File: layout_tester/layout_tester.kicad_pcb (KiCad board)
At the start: 2 copper layers, 178.4 x 118.1 mm, 31 parts, among them SW1 SW_Push

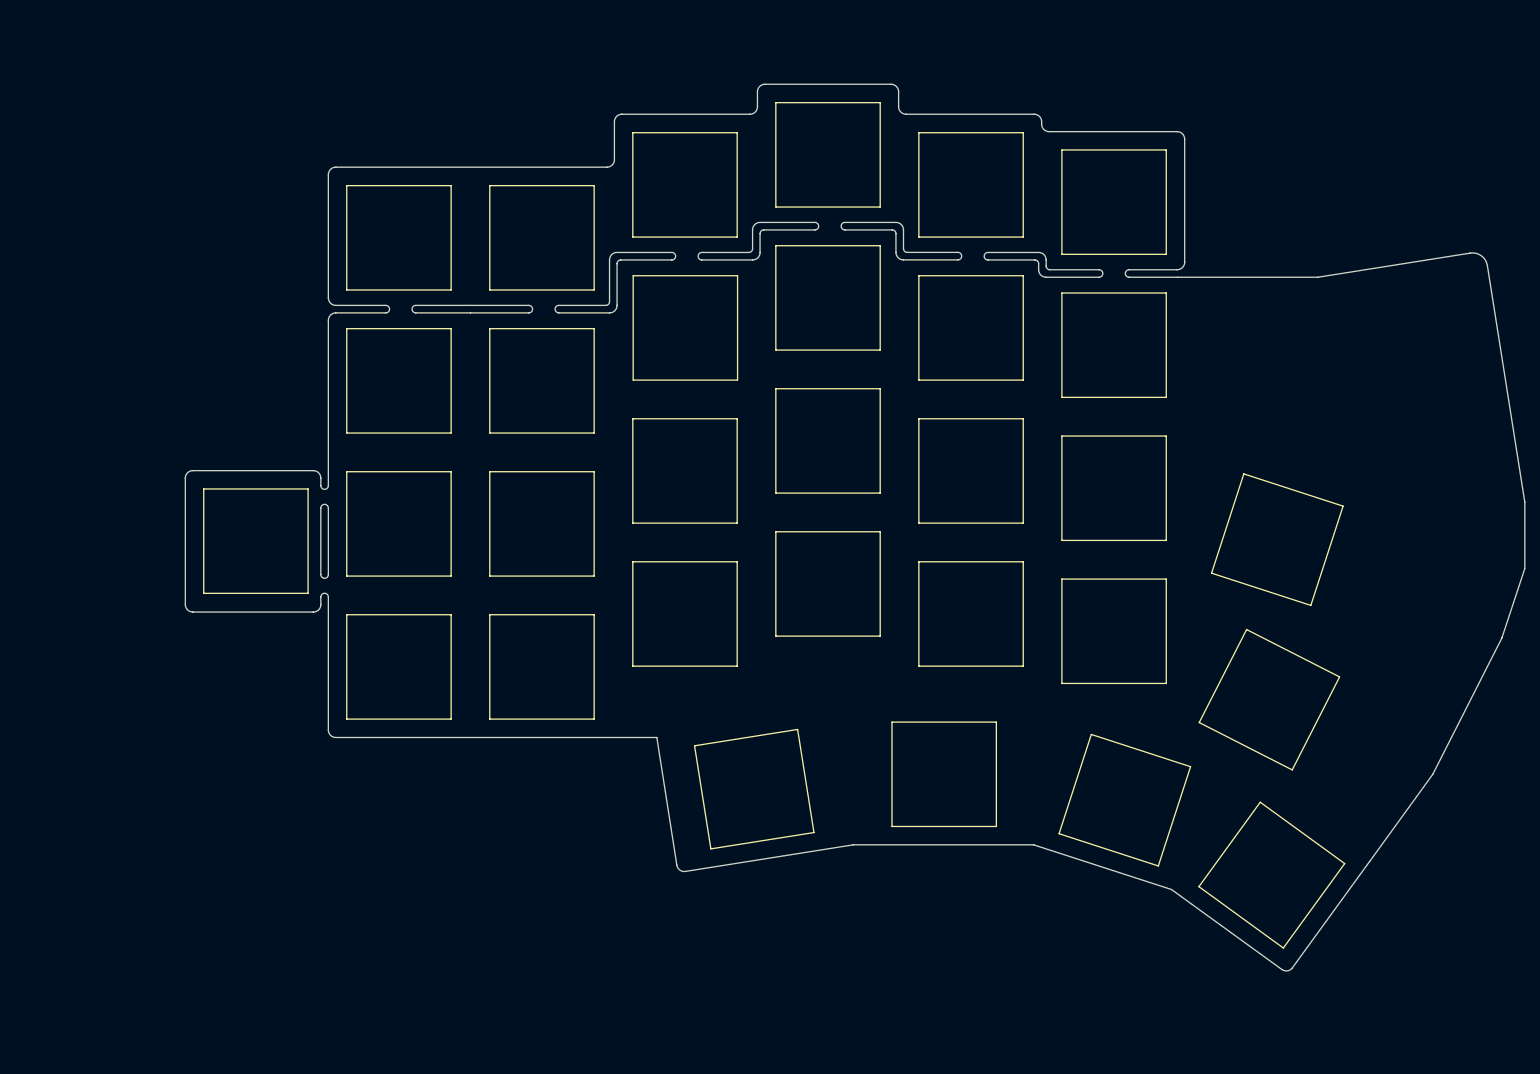
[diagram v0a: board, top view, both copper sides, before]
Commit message: Layout tester
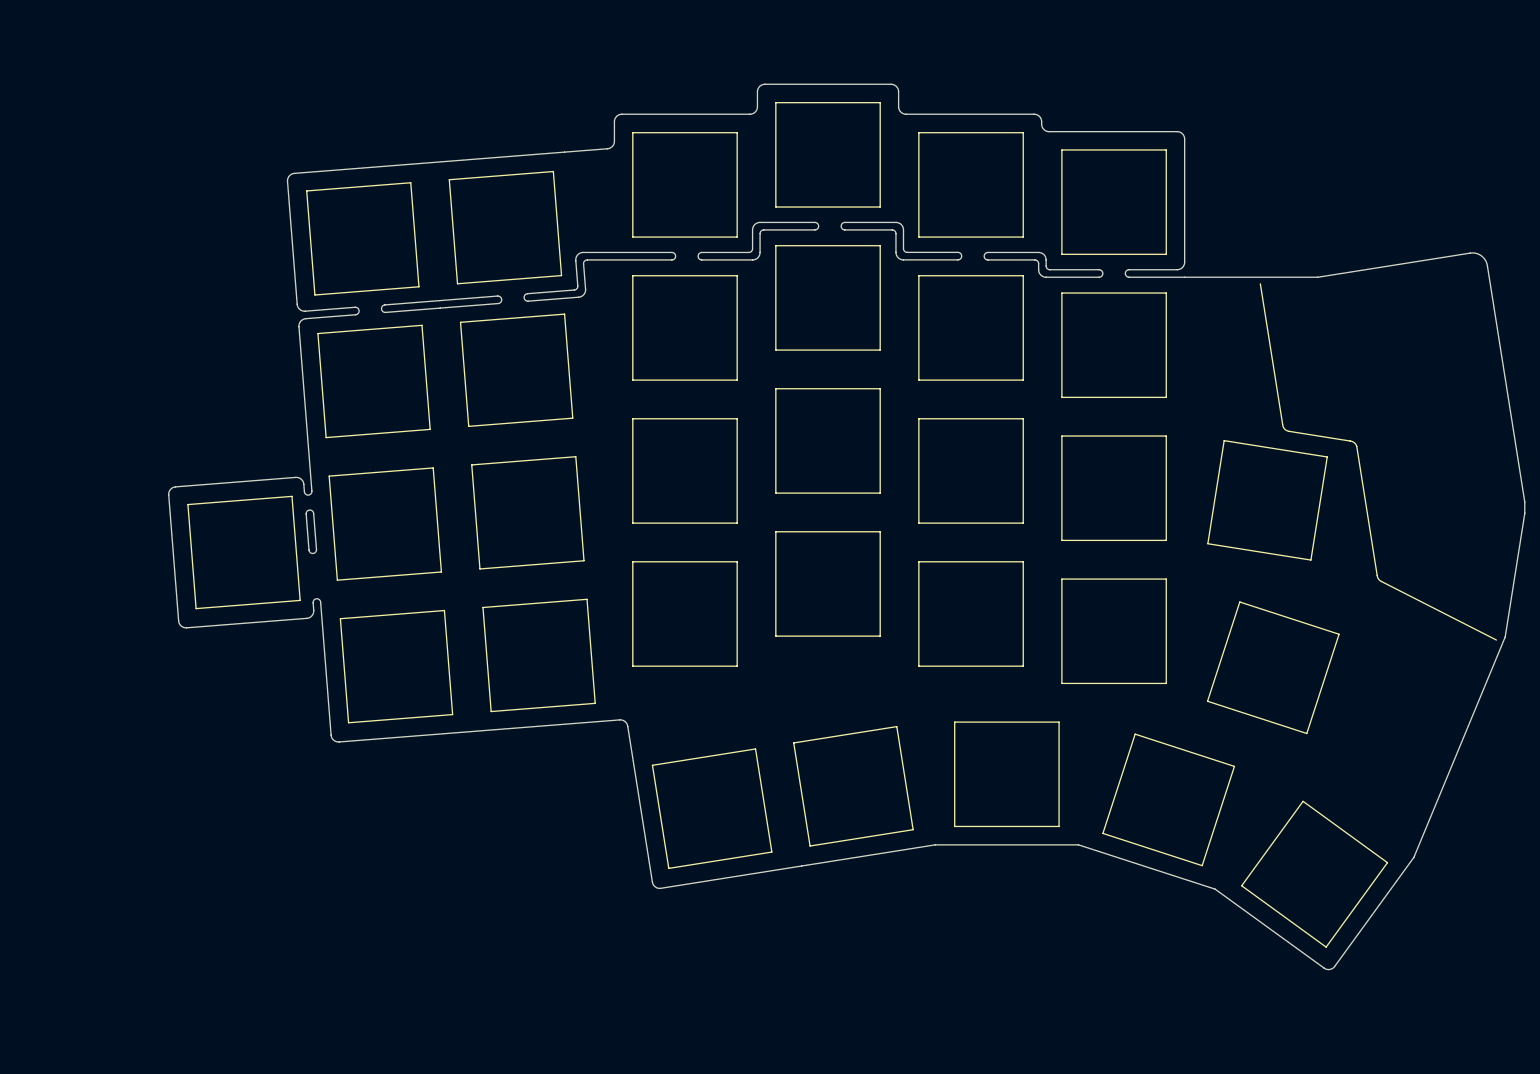
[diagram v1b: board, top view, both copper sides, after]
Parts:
- removed the SW1 at (181.2, 63.0)
- removed the SW1 at (200.2, 103.4)
- removed the SW1 at (200.2, 46.2)
- removed the SW1 at (162.2, 40.0)
- removed the SW1 at (124.0, 108.2)
- removed the SW1 at (143.2, 63.0)
- removed the SW1 at (143.1, 101.1)
- removed the SW1 at (143.1, 82.0)
- removed the SW1 at (181.2, 101.1)
- removed the SW1 at (181.2, 44.0)
- removed the SW1 at (86.0, 91.4)
- removed the SW1 at (162.2, 78.0)
- removed the SW1 at (124.0, 70.0)
- removed the SW1 at (105.0, 51.0)
- removed the SW1 at (124.0, 89.1)
- removed the SW1 at (162.2, 59.0)
- removed the SW1 at (124.0, 51.0)
- removed the SW1 at (105.0, 70.0)
- removed the SW1 at (177.6, 122.5)
- removed the SW1 at (201.7, 125.9)
- removed the SW1 at (220.9, 112.5)
- removed the SW1 at (152.3, 124.4)
- removed the SW1 at (105.0, 108.2)
- removed the SW1 at (222.0, 91.2)
- removed the SW1 at (105.0, 89.1)
- removed the SW1 at (143.1, 44.0)
- removed the SW1 at (162.2, 97.1)
- removed the SW1 at (181.2, 82.0)
- removed the SW1 at (221.3, 135.9)
- removed the SW1 at (200.2, 65.3)
- removed the SW1 at (200.2, 84.3)
- added SW1: SW_Push, used_footprints:CherryMX_Hole_for_layout_tester, F.Cu at (100.2, 51.1)
- added SW10: SW_Push, used_footprints:CherryMX_Hole_for_layout_tester, F.Cu at (162.2, 59.0)
- added SW11: SW_Push, used_footprints:CherryMX_Hole_for_layout_tester, F.Cu at (181.2, 63.0)
- added SW12: SW_Push, used_footprints:CherryMX_Hole_for_layout_tester, F.Cu at (200.2, 65.3)
- added SW13: SW_Push, used_footprints:CherryMX_Hole_for_layout_tester, F.Cu at (103.2, 89.1)
- added SW14: SW_Push, used_footprints:CherryMX_Hole_for_layout_tester, F.Cu at (122.2, 87.6)
- added SW15: SW_Push, used_footprints:CherryMX_Hole_for_layout_tester, F.Cu at (143.1, 82.0)
- added SW16: SW_Push, used_footprints:CherryMX_Hole_for_layout_tester, F.Cu at (162.2, 78.0)
- added SW17: SW_Push, used_footprints:CherryMX_Hole_for_layout_tester, F.Cu at (181.2, 82.0)
- added SW18: SW_Push, used_footprints:CherryMX_Hole_for_layout_tester, F.Cu at (200.2, 84.3)
- added SW19: SW_Push, used_footprints:CherryMX_Hole_for_layout_tester, F.Cu at (220.7, 86.0)
- added SW2: SW_Push, used_footprints:CherryMX_Hole_for_layout_tester, F.Cu at (119.2, 49.6)
- added SW20: SW_Push, used_footprints:CherryMX_Hole_for_layout_tester, F.Cu at (104.7, 108.1)
- added SW21: SW_Push, used_footprints:CherryMX_Hole_for_layout_tester, F.Cu at (123.7, 106.6)
- added SW22: SW_Push, used_footprints:CherryMX_Hole_for_layout_tester, F.Cu at (143.1, 101.1)
- added SW23: SW_Push, used_footprints:CherryMX_Hole_for_layout_tester, F.Cu at (162.2, 97.1)
- added SW24: SW_Push, used_footprints:CherryMX_Hole_for_layout_tester, F.Cu at (181.2, 101.1)
- added SW25: SW_Push, used_footprints:CherryMX_Hole_for_layout_tester, F.Cu at (200.2, 103.4)
- added SW26: SW_Push, used_footprints:CherryMX_Hole_for_layout_tester, F.Cu at (221.5, 108.3)
- added SW27: SW_Push, used_footprints:CherryMX_Hole_for_layout_tester, F.Cu at (84.4, 92.9)
- added SW28: SW_Push, used_footprints:CherryMX_Hole_for_layout_tester, F.Cu at (146.7, 127.0)
- added SW29: SW_Push, used_footprints:CherryMX_Hole_for_layout_tester, F.Cu at (165.5, 124.1)
- added SW3: SW_Push, used_footprints:CherryMX_Hole_for_layout_tester, F.Cu at (143.1, 44.0)
- added SW30: SW_Push, used_footprints:CherryMX_Hole_for_layout_tester, F.Cu at (186.0, 122.5)
- added SW31: SW_Push, used_footprints:CherryMX_Hole_for_layout_tester, F.Cu at (207.5, 125.9)
- added SW32: SW_Push, used_footprints:CherryMX_Hole_for_layout_tester, F.Cu at (227.0, 135.8)
- added SW4: SW_Push, used_footprints:CherryMX_Hole_for_layout_tester, F.Cu at (162.2, 40.0)
- added SW5: SW_Push, used_footprints:CherryMX_Hole_for_layout_tester, F.Cu at (181.2, 44.0)
- added SW6: SW_Push, used_footprints:CherryMX_Hole_for_layout_tester, F.Cu at (200.2, 46.2)
- added SW7: SW_Push, used_footprints:CherryMX_Hole_for_layout_tester, F.Cu at (101.7, 70.1)
- added SW8: SW_Push, used_footprints:CherryMX_Hole_for_layout_tester, F.Cu at (120.7, 68.6)
- added SW9: SW_Push, used_footprints:CherryMX_Hole_for_layout_tester, F.Cu at (143.1, 63.0)
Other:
- board size 178.4 x 118.1 mm -> 180.6 x 117.9 mm

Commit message: Updated the layout tester
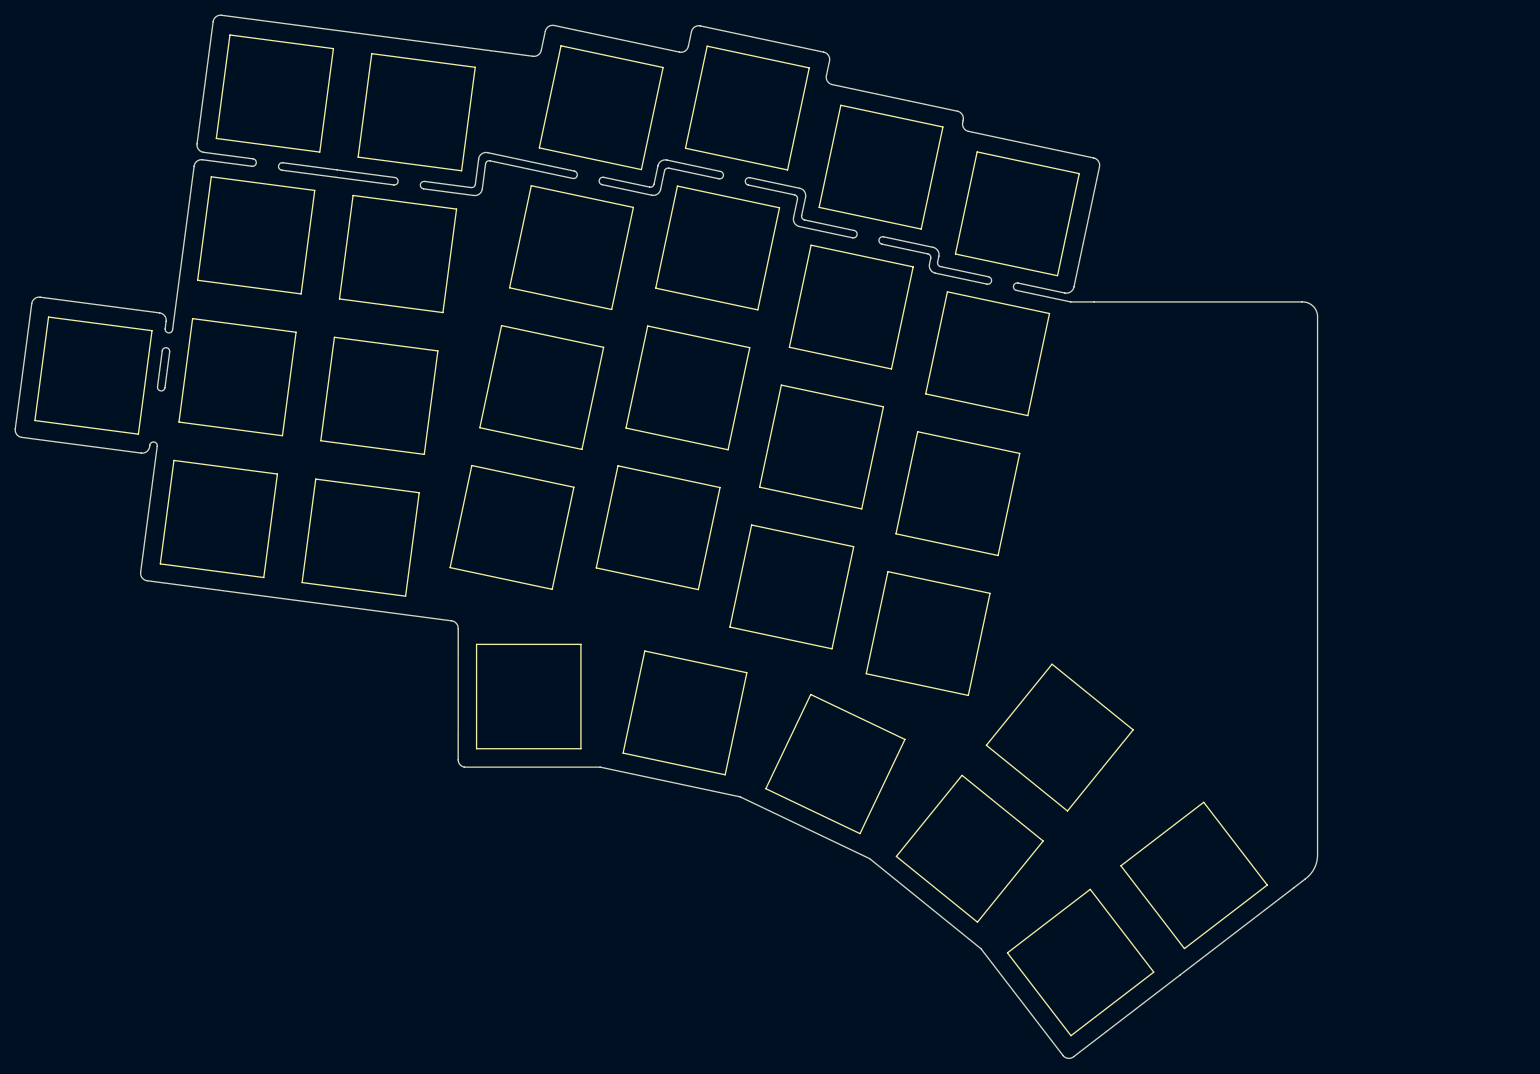
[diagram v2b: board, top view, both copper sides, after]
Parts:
- moved SW19 50.9 mm to (210.9, 135.9), turned to 127.5 degrees
- moved SW32 33.3 mm to (195.8, 147.5), turned to 307.5 degrees
- moved SW27 30.9 mm to (64.3, 69.4), turned to 172.5 degrees
- moved SW20 30.8 mm to (81.0, 88.4), turned to 172.5 degrees
- moved SW26 29.9 mm to (193.0, 117.6), turned to 141 degrees
- moved SW28 28.6 mm to (122.3, 112.1), turned to 0 degrees
- moved SW21 28.5 mm to (99.9, 90.9), turned to 172.5 degrees
- moved SW13 27.7 mm to (83.5, 69.6), turned to 172.5 degrees
- moved SW31 27.3 mm to (181.0, 132.4), turned to 321 degrees
- moved SW22 25.8 mm to (120.1, 89.6), turned to 168 degrees
- moved SW14 25.2 mm to (102.4, 72.0), turned to 172.5 degrees
- moved SW7 25.0 mm to (86.0, 50.7), turned to 172.5 degrees
- moved SW25 24.8 mm to (175.5, 103.7), turned to 168 degrees
- moved SW29 24.5 mm to (143.1, 114.3), turned to 348 degrees
- moved SW24 24.1 mm to (157.3, 97.5), turned to 168 degrees
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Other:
- board size 180.6 x 117.9 mm -> 173.5 x 138.9 mm
